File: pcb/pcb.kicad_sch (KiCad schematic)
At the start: 239 parts, among them SW1 SW_DIP_x01_XKB_TS_2030, SW2 SW_DIP_x01_XKB_TS_2030, U1 RP2040, U2 Memory_Flash_W25Q64_XSON, U3 NCP114ASN330T1G, X1 12.000MHz

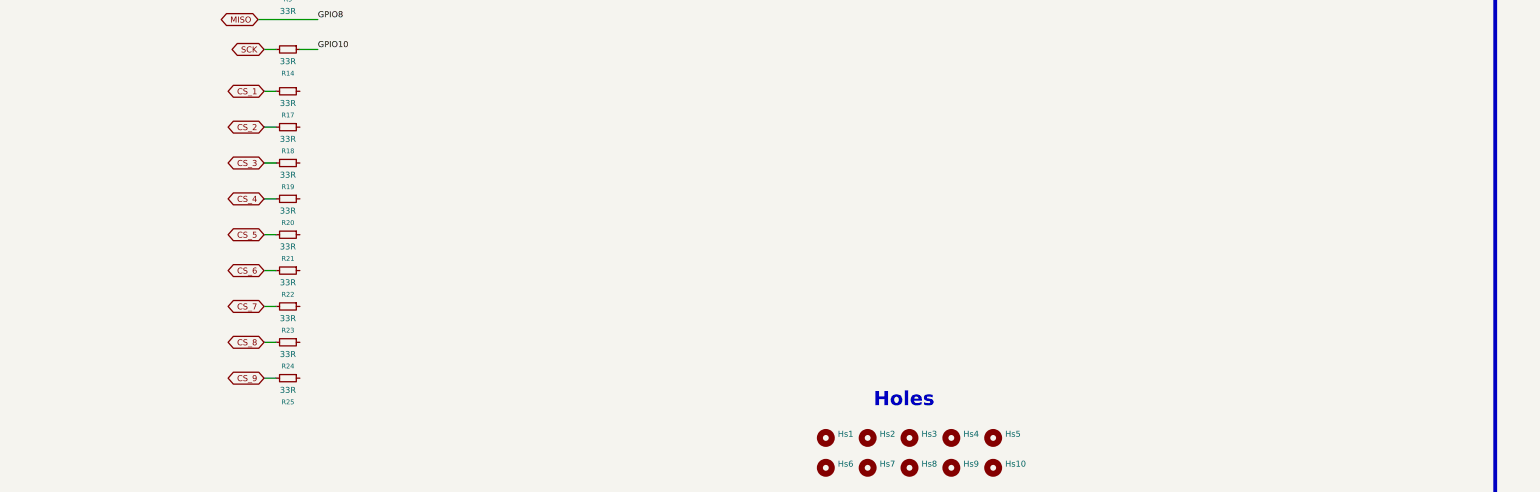
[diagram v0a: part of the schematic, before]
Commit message: M  notes/spi M  pcb/pcb.kicad_pcb M  pcb/pcb.kicad_sch M  placefp.py A  tracks.py
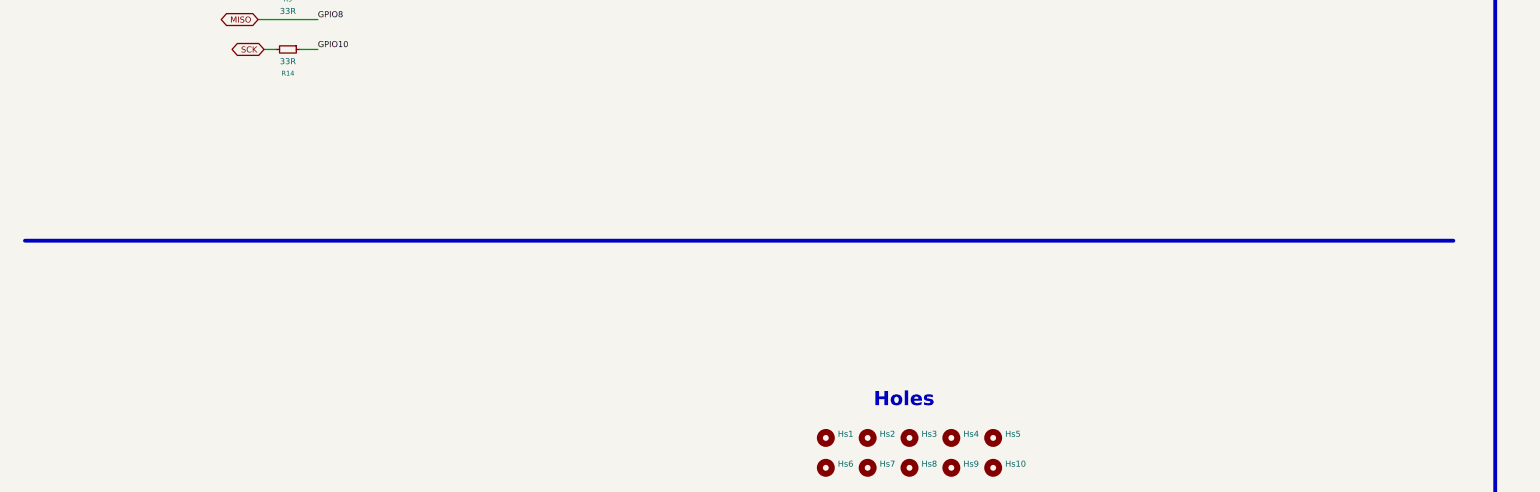
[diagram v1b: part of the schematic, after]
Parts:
- removed R17, R18, R19, R20, R21, R22, R23, R24, R25: 33R, tmr-lib:R_0603_1608Metric, symbol Device:R_Small
